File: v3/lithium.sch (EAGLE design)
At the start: 60 parts, among them J1 batt, J2 battery, J3 motor, J4 AVR_ISP, Q1 Si7137DP, Q1_R1 100k, U1 TPS61088VQFN20, U1_C22 8.2nF, U1_CBST 100nF, U1_CCOMP 680PF, U1_CCOMP2 36pF, U1_CIN 0.47uF, U1_CIN2 100nF, U1_COUT 0.47uF, U1_CVCC 1uF, U1_L1 DR73-1R0-R, U1_RCOMP 38.3K Ohms, U1_RFBB 118K Ohms, U1_RFBT 470K Ohms, U1_RLIM 102K Ohms, U1_RT 261K Ohms, U2 ATTINY84-20MU, U2_C1 22uF, U2_C2 22uF, U2_R1 10k, U2_R2 10k, U4 TPS2113APWR, U4_C3 0.1uF, U4_C4 0.1uF, U4_RPG 100K Ohms, U5 MCP73833-FCI/UN, U5_C1 1.0uF, U5_C2 1.0uF, U5_R1 1K Ohm, U6 TPS61230A, U6_CBST 10 nF, U6_CFF 10pF, U6_CIN 22uF, U6_COUT 22uF, U6_RFBB 100K Ohms, U6_RFBT 316K Ohms

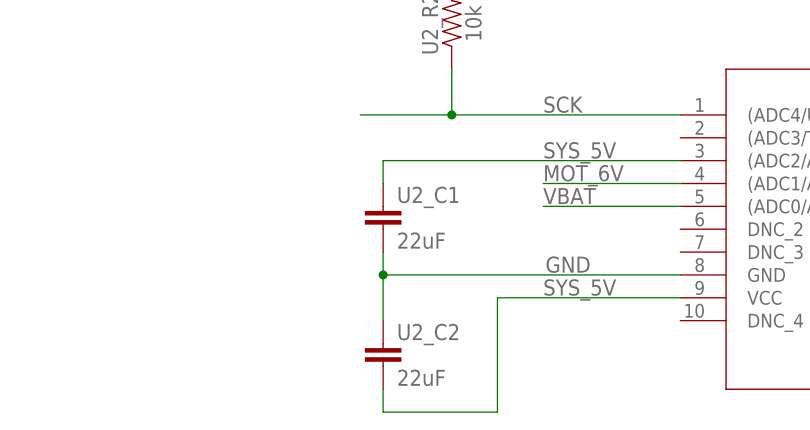
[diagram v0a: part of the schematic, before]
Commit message: Okay, I think this fixed it.
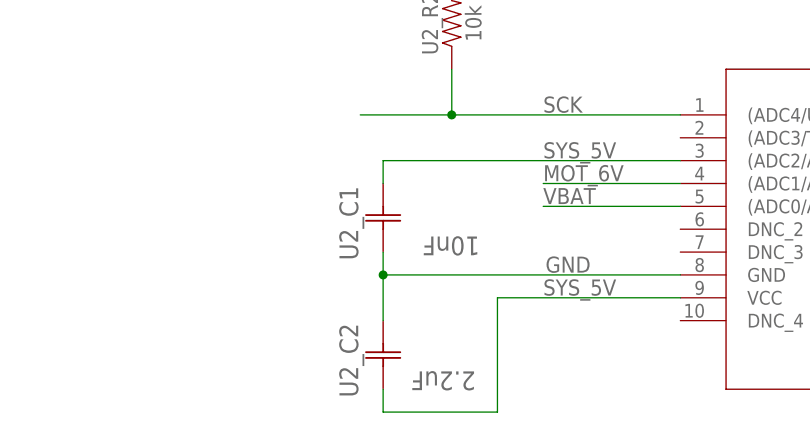
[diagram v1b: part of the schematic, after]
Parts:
- U2_C1: value 22uF -> 10nF; device 32bits:CAPACITOR0402 -> Yageo_By_element14_Batch_1:CC0402KRX7R7BB103
- U2_C2: value 22uF -> 2.2uF; device 32bits:CAPACITOR0402 -> AVX_By_element14_Batch_1:0402ZD225KAT2A
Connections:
- net GND: now also U2_C1.C1, U2_C2.C2; no longer U2_C1.2, U2_C2.1
- net SYS_5V: now also U2_C1.C2, U2_C2.C1; no longer U2_C1.1, U2_C2.2
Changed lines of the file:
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@@
 <part name="J4" library="32bits" deviceset="AVR_ISP" device=""/>
 <part name="U4_RPG" library="Vishay_By_element14_Batch_1" deviceset="CRCW1206100KFKEA" device="" value="100K Ohms"/>
-<part name="U2_C1" library="32bits" deviceset="CAPACITOR" device="0402" value="22uF"/>
-<part name="U2_C2" library="32bits" deviceset="CAPACITOR" device="0402" value="22uF"/>
 <part name="Q1_R1" library="SparkFun-Resistors" deviceset="100KOHM" device="-0603-1/10W-1%" value="100k"/>
 <part name="D1" library="SparkFun-DiscreteSemi" deviceset="DIODE-SCHOTTKY" device="-BAT20J" value="1SS367,H3F"/>
 <part name="U2_R2" library="SparkFun-Resistors" deviceset="RESISTOR" device="0402" value="10k"/>
 <part name="U2_R1" library="SparkFun-Resistors" deviceset="RESISTOR" device="0402" value="10k"/>
+<part name="U2_C1" library="Yageo_By_element14_Batch_1" deviceset="CC0402KRX7R7BB103" device="" value="10nF"/>
+<part name="U2_C2" library="AVX_By_element14_Batch_1" deviceset="0402ZD225KAT2A" device="" value="2.2uF"/>
 </parts>
 <sheets>
@@
 <instance part="J4" gate="A" x="-12.7" y="213.36"/>
 <instance part="U4_RPG" gate="A" x="292.1" y="53.34" rot="R90"/>
-<instance part="U2_C1" gate="G$1" x="5.08" y="-48.26"/>
-<instance part="U2_C2" gate="G$1" x="5.08" y="-63.5"/>
 <instance part="Q1_R1" gate="G$1" x="-33.02" y="241.3"/>
 <instance part="D1" gate="G$1" x="-22.86" y="233.68" rot="R270"/>
 <instance part="U2_R2" gate="G$1" x="12.7" y="-27.94" rot="R90"/>
 <instance part="U2_R1" gate="G$1" x="236.22" y="-43.18" rot="R90"/>
+<instance part="U2_C1" gate="A" x="5.08" y="-53.34" smashed="yes" rot="R90">
+<attribute name="VALUE" x="15.8242" y="-51.6128" size="2.0828" layer="96" ratio="10" rot="SR180"/>
+<attribute name="NAME" x="2.3114" y="-54.2544" size="2.0828" layer="95" ratio="10" rot="SR90"/>
+</instance>
+<instance part="U2_C2" gate="A" x="5.08" y="-68.58" smashed="yes" rot="R90">
+<attribute name="VALUE" x="15.367" y="-66.5988" size="2.0828" layer="96" ratio="10" rot="SR180"/>
+<attribute name="NAME" x="2.3114" y="-69.4944" size="2.0828" layer="95" ratio="10" rot="SR90"/>
+</instance>
 </instances>
 <busses>
@@
 <pinref part="U2" gate="A" pin="GND"/>
 <label x="23.114" y="-55.626" size="1.778" layer="95"/>
-<pinref part="U2_C1" gate="G$1" pin="2"/>
 <wire x1="38.1" y1="-55.88" x2="5.08" y2="-55.88" width="0.1524" layer="91"/>
 <wire x1="5.08" y1="-55.88" x2="5.08" y2="-53.34" width="0.1524" layer="91"/>
-<pinref part="U2_C2" gate="G$1" pin="1"/>
 <wire x1="5.08" y1="-60.96" x2="5.08" y2="-55.88" width="0.1524" layer="91"/>
 <junction x="5.08" y="-55.88"/>
+<pinref part="U2_C1" gate="A" pin="C1"/>
+<pinref part="U2_C2" gate="A" pin="C2"/>
 </segment>
 <segment>
@@
 <wire x1="17.78" y1="-58.42" x2="17.78" y2="-71.12" width="0.1524" layer="91"/>
 <wire x1="17.78" y1="-71.12" x2="5.08" y2="-71.12" width="0.1524" layer="91"/>
-<pinref part="U2_C2" gate="G$1" pin="2"/>
 <wire x1="5.08" y1="-71.12" x2="5.08" y2="-68.58" width="0.1524" layer="91"/>
+<pinref part="U2_C2" gate="A" pin="C1"/>
 </segment>
 <segment>
 <pinref part="U2" gate="A" pin="(ADC2/AIN1/PCINT2)_PA2"/>
 <label x="22.86" y="-42.926" size="1.778" layer="95"/>
-<pinref part="U2_C1" gate="G$1" pin="1"/>
 <wire x1="38.1" y1="-43.18" x2="5.08" y2="-43.18" width="0.1524" layer="91"/>
 <wire x1="5.08" y1="-43.18" x2="5.08" y2="-45.72" width="0.1524" layer="91"/>
-</segment>
-<segment>
+<pinref part="U2_C1" gate="A" pin="C2"/>
+</segment>
+<segment>

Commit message: Release candidate.
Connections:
- net LOCAL_VBAT renamed VBAT_JST
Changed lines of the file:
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@@
 </segment>
 </net>
-<net name="LOCAL_VBAT" class="0">
+<net name="VBAT_JST" class="0">
 <segment>
 <pinref part="J1" gate="G$1" pin="1"/>
